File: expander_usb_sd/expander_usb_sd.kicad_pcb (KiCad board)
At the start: 2 copper layers, 59.7 x 128.5 mm, 10 parts, among them J1 Micro_SD_Card_Det1, J1-TeensyPower1 USB power - Teensy device, J2 Internal_USB_Host_Teensy, J5-TeensyMicroUSB1 USB 5 pin to Teensy/MicroUSB, J6-USBHost1 USB 5 pin to frontpanel/Type C

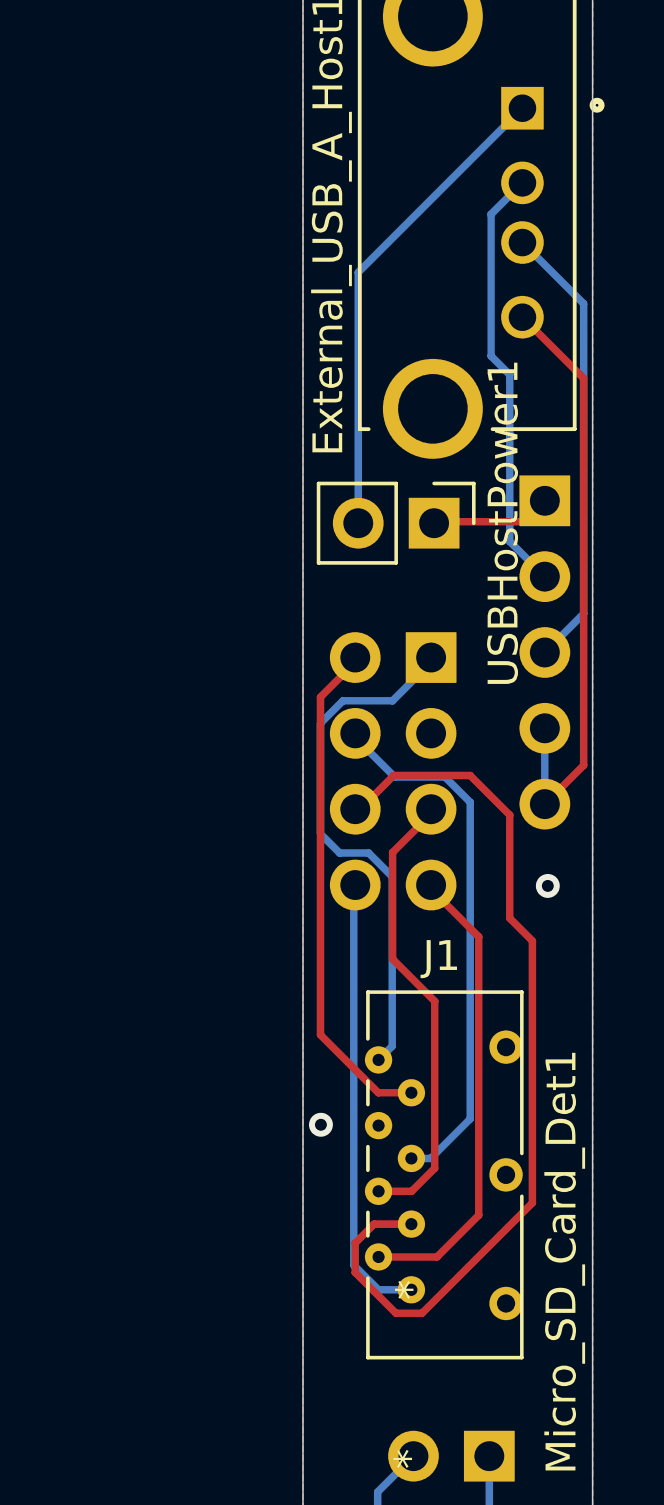
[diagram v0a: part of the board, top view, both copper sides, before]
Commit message: believe fixed problems with expander_usb_sd; tracked a bunch of stuff that was untracked (expander_cv_output?)
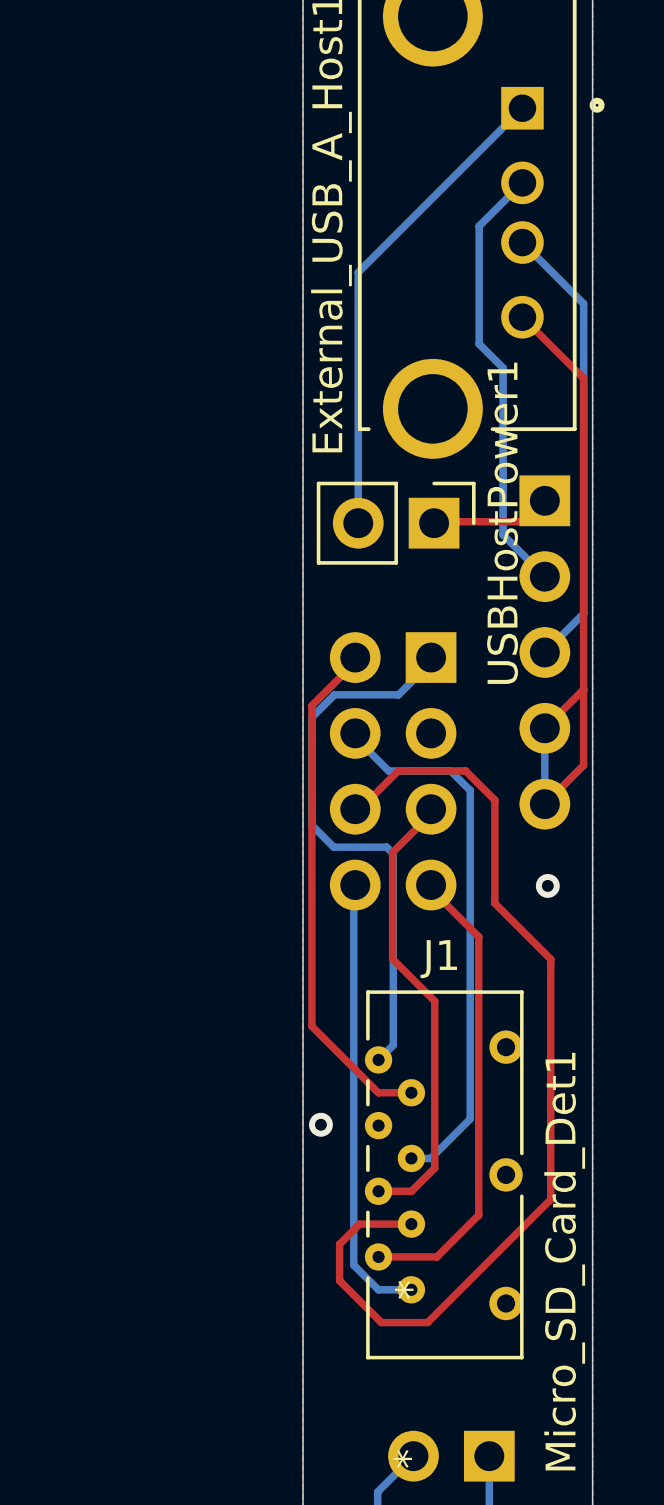
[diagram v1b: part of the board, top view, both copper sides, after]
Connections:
- J2 pad 4: Net-(External_USB_A_Host1-SHIELD) -> Net-(External_USB_A_Host1-GND)
- J2 pad 5: Net-(External_USB_A_Host1-SHIELD) -> Net-(External_USB_A_Host1-GND)
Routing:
- net /CMD: track 30.7 -> 33.1 mm
- net Net-(External_USB_A_Host1-GND): track 20.2 -> 22.1 mm
- net /DAT1: track 17.6 -> 18.6 mm
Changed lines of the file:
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@@
 	(net 19 "Net-(J5-TeensyMicroUSB1-Pin_4)")
 	(net 20 "Net-(J5-TeensyMicroUSB1-Pin_5)")
-	(net 21 "Net-(External_USB_A_Host1-SHIELD)")
 	(footprint "footprints:PJS008U-3000-0"
 		(layer "F.Cu")
@@
 		(tags "Through hole pin header THT 1x05 2.54mm single row")
 		(property "Reference" "J5-TeensyMicroUSB1"
-			(at 0 2.33 0)
+			(at -2 -4.6 90)
 			(layer "B.SilkS")
 			(effects
@@
 		(tags "Through hole pin header THT 1x02 2.54mm single row")
 		(property "Reference" "J1-TeensyPower1"
-			(at 0 2.33 90)
+			(at -1.975 0.01 180)
 			(layer "B.SilkS")
 			(effects
@@
 		(tags "Through hole pin header THT 1x05 2.54mm single row")
 		(property "Reference" "J6-USBHost1"
-			(at 0 2.33 0)
+			(at 1.925 -4.99 90)
 			(layer "B.SilkS")
 			(effects
@@
 			(layers "*.Cu" "*.Mask")
 			(remove_unused_layers no)
-			(net 21 "Net-(External_USB_A_Host1-SHIELD)")
+			(net 4 "Net-(External_USB_A_Host1-GND)")
 			(pinfunction "Pin_4")
 			(pintype "passive")
@@
 			(layers "*.Cu" "*.Mask")
 			(remove_unused_layers no)
-			(net 21 "Net-(External_USB_A_Host1-SHIELD)")
+			(net 4 "Net-(External_USB_A_Host1-GND)")
 			(pinfunction "Pin_5")
 			(pintype "passive")
@@
 		(tags "Through hole pin header THT 2x04 2.54mm double row")
 		(property "Reference" "SD_connector1"
-			(at 1.27 2.33 0)
+			(at 7.39 2.025 0)
 			(layer "B.SilkS")
 			(effects
@@
 	)
 	(segment
-		(start 131.225 72.075)
-		(end 130.6 71.45)
+		(start 130.2 71.05)
+		(end 130.2 67.1)
 		(width 0.25)
 		(layer "B.Cu")
@@
 	)
 	(segment
-		(start 131.225 77.665)
-		(end 131.225 72.075)
+		(start 131 77.44)
+		(end 131 71.85)
 		(width 0.25)
 		(layer "B.Cu")
@@
 	(segment
 		(start 132.4 78.84)
-		(end 131.225 77.665)
+		(end 131 77.44)
 		(width 0.25)
 		(layer "B.Cu")
@@
 	)
 	(segment
-		(start 130.6 66.7)
+		(start 130.2 67.1)
 		(end 131.65 65.65)
 		(width 0.25)
@@
 	)
 	(segment
-		(start 130.6 71.45)
-		(end 130.6 66.7)
+		(start 131 71.85)
+		(end 130.2 71.05)
 		(width 0.25)
 		(layer "B.Cu")
@@
 	)
 	(segment
-		(start 133.7 85.16)
+		(start 133.7 82.625)
 		(end 133.7 72.2)
 		(width 0.25)
@@
 	)
 	(segment
+		(start 133.7 85.16)
+		(end 133.7 82.625)
+		(width 0.25)
+		(layer "F.Cu")
+		(net 4)
+	)
+	(segment
+		(start 133.7 85.16)
+		(end 132.4 86.46)
+		(width 0.25)
+		(layer "F.Cu")
+		(net 4)
+	)
+	(segment
 		(start 133.7 72.2)
 		(end 131.65 70.15)
@@
 	)
 	(segment
-		(start 132.4 86.46)
-		(end 133.7 85.16)
+		(start 132.4 83.92)
+		(end 133.695 82.625)
+		(width 0.25)
+		(layer "F.Cu")
+		(net 4)
+	)
+	(segment
+		(start 133.695 82.625)
+		(end 133.7 82.625)
 		(width 0.25)
 		(layer "F.Cu")
@@
 	)
 	(segment
-		(start 124.885 94.189199)
-		(end 124.885 82.875)
+		(start 127.929999 96.128001)
+		(end 126.823802 96.128001)
 		(width 0.25)
 		(layer "F.Cu")
@@
 	)
 	(segment
-		(start 124.885 82.875)
+		(start 124.6 83.16)
 		(end 126.06 81.7)
 		(width 0.25)
@@
 	)
 	(segment
-		(start 126.823802 96.128001)
-		(end 124.885 94.189199)
+		(start 124.6 93.904199)
+		(end 124.6 83.16)
 		(width 0.25)
 		(layer "F.Cu")
@@
 	)
 	(segment
-		(start 127.929999 96.128001)
-		(end 126.823802 96.128001)
+		(start 126.823802 96.128001)
+		(end 124.6 93.904199)
 		(width 0.25)
 		(layer "F.Cu")
@@
 	)
 	(segment
-		(start 131.9838 99.8162)
-		(end 131.9838 91.042099)
+		(start 130.725 89.783299)
+		(end 130.725 86.325)
 		(width 0.25)
 		(layer "F.Cu")
@@
 	)
 	(segment
-		(start 126.047799 101.1624)
-		(end 126.047799 102.147799)
+		(start 126.925 103.825)
+		(end 128.475 103.825)
 		(width 0.25)
 		(layer "F.Cu")
@@
 	)
 	(segment
-		(start 131.9838 91.042099)
-		(end 131.225 90.283299)
+		(start 132.6 91.658299)
+		(end 130.725 89.783299)
 		(width 0.25)
 		(layer "F.Cu")
@@
 	)
 	(segment
-		(start 131.225 86.825)
-		(end 129.9 85.5)
+		(start 129.75 85.35)
+		(end 127.49 85.35)
 		(width 0.25)
 		(layer "F.Cu")
@@
 	)
 	(segment
-		(start 128.2898 103.5102)
-		(end 131.9838 99.8162)
+		(start 125.525 102.425)
+		(end 126.925 103.825)
 		(width 0.25)
 		(layer "F.Cu")
@@
 	)
 	(segment
-		(start 127.929999 100.527999)
-		(end 126.6822 100.527999)
+		(start 126.197001 100.527999)
+		(end 125.525 101.2)
 		(width 0.25)
 		(layer "F.Cu")
@@
 	)
 	(segment
-		(start 126.047799 102.147799)
-		(end 127.4102 103.5102)
+		(start 132.6 99.7)
+		(end 132.6 91.658299)
 		(width 0.25)
 		(layer "F.Cu")
@@
 	)
 	(segment
-		(start 129.9 85.5)
-		(end 127.34 85.5)
+		(start 125.525 101.2)
+		(end 125.525 102.425)
 		(width 0.25)
 		(layer "F.Cu")
@@
 	)
 	(segment
-		(start 127.34 85.5)
-		(end 126.06 86.78)
+		(start 128.475 103.825)
+		(end 132.6 99.7)
 		(width 0.25)
 		(layer "F.Cu")
@@
 	)
 	(segment
-		(start 126.6822 100.527999)
-		(end 126.047799 101.1624)
+		(start 127.929999 100.527999)
+		(end 126.197001 100.527999)
 		(width 0.25)
 		(layer "F.Cu")
@@
 	)
 	(segment
-		(start 131.225 90.283299)
-		(end 131.225 86.825)
+		(start 127.49 85.35)
+		(end 126.06 86.78)
 		(width 0.25)
 		(layer "F.Cu")
@@
 	)
 	(segment
-		(start 127.4102 103.5102)
-		(end 128.2898 103.5102)
+		(start 130.725 86.325)
+		(end 129.75 85.35)
 		(width 0.25)
 		(layer "F.Cu")
@@
 	)
 	(segment
-		(start 129.9 86.4)
-		(end 129.9 97.004578)
+		(start 129.25 85.35)
+		(end 129.9 86)
 		(width 0.25)
 		(layer "B.Cu")
@@
 	)
 	(segment
-		(start 128.576577 98.328001)
-		(end 127.929999 98.328001)
+		(start 129.9 86)
+		(end 129.9 97.004578)
 		(width 0.25)
 		(layer "B.Cu")
@@
 	)
 	(segment
-		(start 127.37 85.55)
-		(end 129.05 85.55)
+		(start 129.9 97.004578)
+		(end 128.576577 98.328001)
 		(width 0.25)
 		(layer "B.Cu")
@@
 	)
 	(segment
-		(start 126.06 84.24)
-		(end 127.37 85.55)
+		(start 127.17 85.35)
+		(end 129.25 85.35)
 		(width 0.25)
 		(layer "B.Cu")
@@
 	)
 	(segment
-		(start 129.05 85.55)
-		(end 129.9 86.4)
+		(start 128.576577 98.328001)
+		(end 127.929999 98.328001)
 		(width 0.25)
 		(layer "B.Cu")
@@
 	)
 	(segment
-		(start 129.9 97.004578)
-		(end 128.576577 98.328001)
+		(start 126.06 84.24)
+		(end 127.17 85.35)
 		(width 0.25)
 		(layer "B.Cu")
@@
 	)
 	(segment
-		(start 127.287199 94.5708)
-		(end 126.829999 95.028)
+		(start 127.1 87.9)
+		(end 127.325 88.125)
 		(width 0.25)
 		(layer "B.Cu")
@@
 	)
 	(segment
-		(start 126.501701 88.1)
-		(end 127.287199 88.885498)
+		(start 127.325 94.532999)
+		(end 126.829999 95.028)
 		(width 0.25)
 		(layer "B.Cu")
@@
 	)
 	(segment
-		(start 128.6 81.7)
-		(end 127.3 83)
+		(start 125.35 82.8)
+		(end 124.6 83.55)
 		(width 0.25)
 		(layer "B.Cu")
@@
 	)
 	(segment
-		(start 127.287199 88.885498)
-		(end 127.287199 94.5708)
+		(start 127.5 82.8)
+		(end 125.35 82.8)
 		(width 0.25)
 		(layer "B.Cu")
@@
 	)
 	(segment
-		(start 127.3 83)
-		(end 125.638299 83)
+		(start 124.6 87.171701)
+		(end 125.328299 87.9)
 		(width 0.25)
 		(layer "B.Cu")
@@
 	)
 	(segment
-		(start 124.885 83.753299)
-		(end 124.885 87.456701)
+		(start 127.325 88.125)
+		(end 127.325 94.532999)
 		(width 0.25)
 		(layer "B.Cu")
@@
 	)
 	(segment
-		(start 125.638299 83)
-		(end 124.885 83.753299)
+		(start 124.6 83.55)
+		(end 124.6 87.171701)
 		(width 0.25)
 		(layer "B.Cu")
@@
 	)
 	(segment
-		(start 125.528299 88.1)
-		(end 126.501701 88.1)
+		(start 125.328299 87.9)
+		(end 127.1 87.9)
 		(width 0.25)
 		(layer "B.Cu")
@@
 	)
 	(segment
-		(start 124.885 87.456701)
-		(end 125.528299 88.1)
+		(start 128.6 81.7)
+		(end 127.5 82.8)
 		(width 0.25)
 		(layer "B.Cu")
